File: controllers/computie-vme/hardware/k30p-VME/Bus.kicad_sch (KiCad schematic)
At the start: 2 parts, among them U16 74HC148, U17 VME64-P1-3R

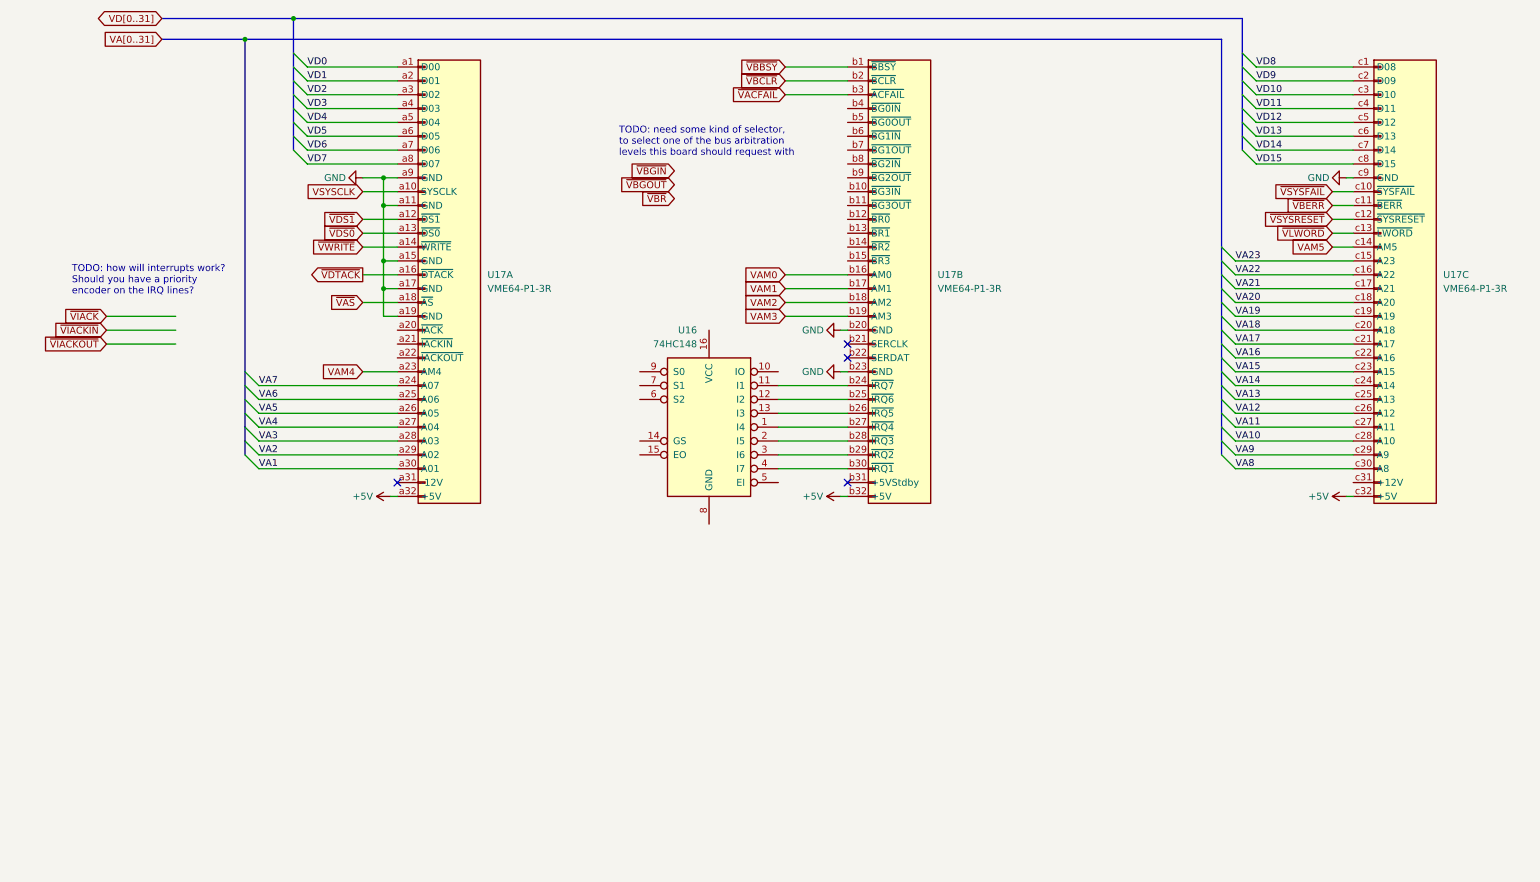
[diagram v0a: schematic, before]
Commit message: Updating with more work in progress
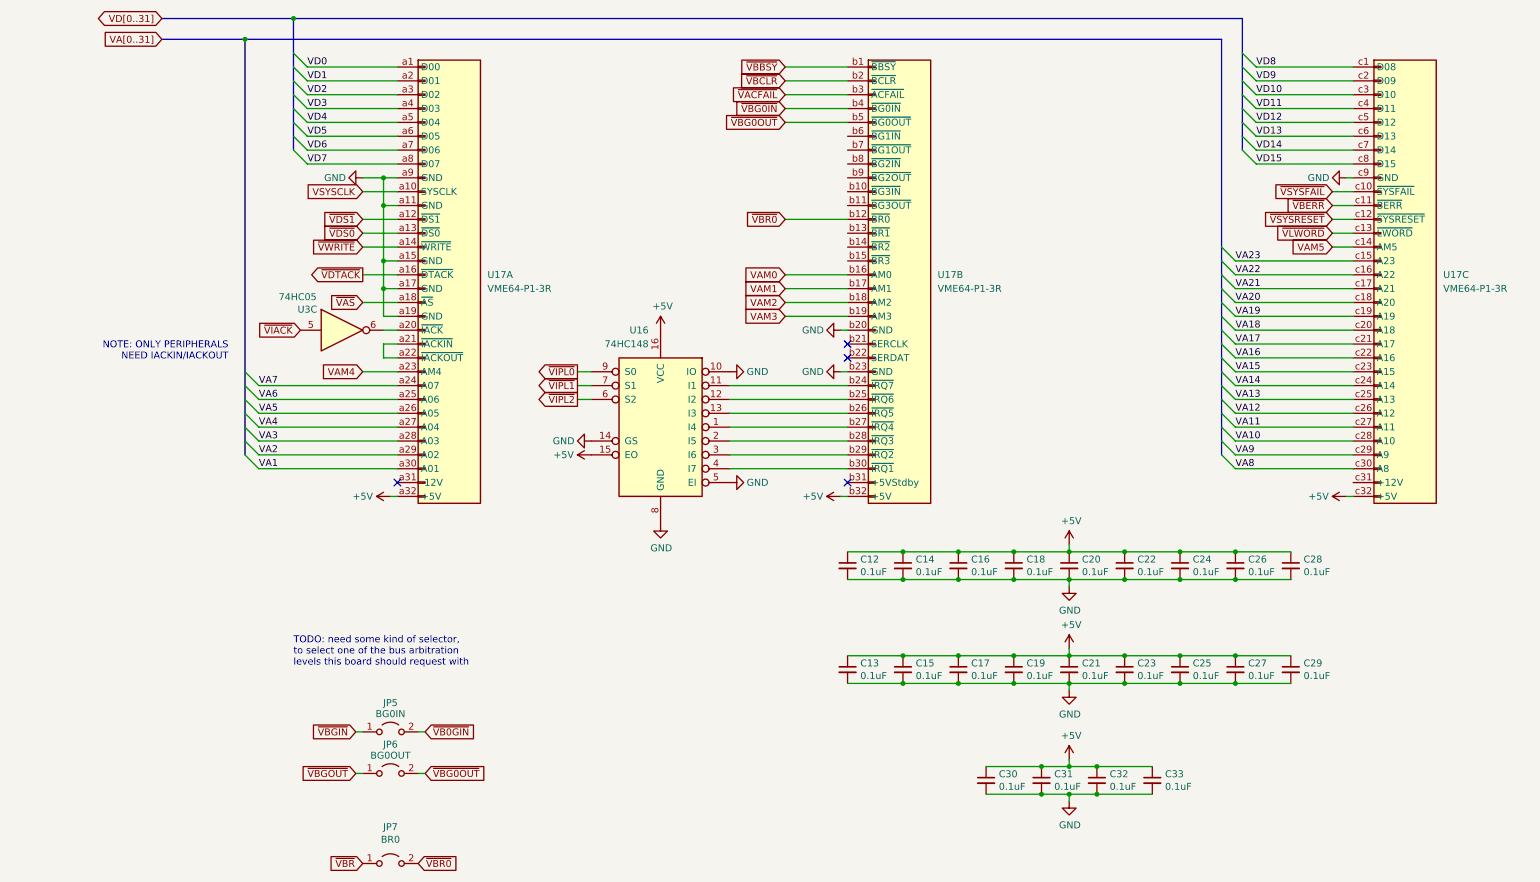
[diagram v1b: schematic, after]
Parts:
- added C12, C13, C14, C15, C16, C17, C18, C19, C20, C21, C22, C23, C24, C25, C26, C27, C28, C29, C30, C31, C32, C33: 0.1uF, Capacitor_SMD:C_0805_2012Metric_Pad1.18x1.45mm_HandSolder, symbol Device:C_Small
- added JP5: BG0IN, Connector_PinHeader_2.54mm:PinHeader_1x02_P2.54mm_Vertical, symbol Jumper:Jumper_2_Open
- added JP6: BG0OUT, Connector_PinHeader_2.54mm:PinHeader_1x02_P2.54mm_Vertical, symbol Jumper:Jumper_2_Open
- added JP7: BR0, Connector_PinHeader_2.54mm:PinHeader_1x02_P2.54mm_Vertical, symbol Jumper:Jumper_2_Open
- added U3: 74HC05, Package_SO:TSSOP-14_4.4x5mm_P0.65mm, symbol 74xx:74LS05
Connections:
- net +5V: now also U16.15 (EO), U16.16 (VCC), C12.1, C13.1, C14.1, C15.1, C16.1, C17.1, C18.1, C19.1, C20.1, C21.1, C22.1, C23.1, C24.1, C25.1, C26.1, C27.1, C28.1, C29.1, C30.1, C31.1, C32.1, C33.1
- net GND: now also U16.10 (IO), U16.14 (GS), U16.5 (EI), U16.8 (GND), C12.2, C13.2, C14.2, C15.2, C16.2, C17.2, C18.2, C19.2, C20.2, C21.2, C22.2, C23.2, C24.2, C25.2, C26.2, C27.2, C28.2, C29.2, C30.2, C31.2, C32.2, C33.2
- net ~{VBGIN}: now also JP5.1 (A)
- net ~{VBGOUT}: now also JP6.1 (A)
- net ~{VBR}: now also JP7.1 (A)
- net ~{VIACK}: now also U3.5
- net ~{VIPL2}: now reaches U16.6 (S2)
- net ~{VIPL1}: now reaches U16.7 (S1)
- net ~{VIPL0}: now reaches U16.9 (S0)
- net ~{VBR0}: now reaches U17.b12 (~{BR0})
- net ~{VBR0}: now also JP7.2 (B)
- net ~{VBG0IN}: now reaches U17.b4 (~{BG0IN})
- net ~{VBG0OUT}: now reaches U17.b5 (~{BG0OUT})
- net ~{VBG0OUT}: now also JP6.2 (B)
- net at U17.a20 (~{IACK}): now also U3.6
- net at U17.a21 (~{IACKIN}): now also U17.a22 (~{IACKOUT})
- new net ~{VB0GIN}: JP5.2 (B)
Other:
- note added: "NOTE: ONLY PERIPHERALS NEED IACKIN/IACKOUT"
- note removed: "TODO: how will interrupts work? Should you have a priority encoder on the IRQ lines?"
- title: k30-VME32 -> k30p-VME
- moved on the sheet: U16
